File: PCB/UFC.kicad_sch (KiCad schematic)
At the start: 73 parts, among them M1 Fan_3pin, M2 Fan_3pin, M3 Fan_3pin, M4 Fan_3pin, M5 Fan_3pin, M6 Fan_3pin, M7 Fan_3pin, M8 Fan_3pin, SW1 PWM 12:5, U1 Pico

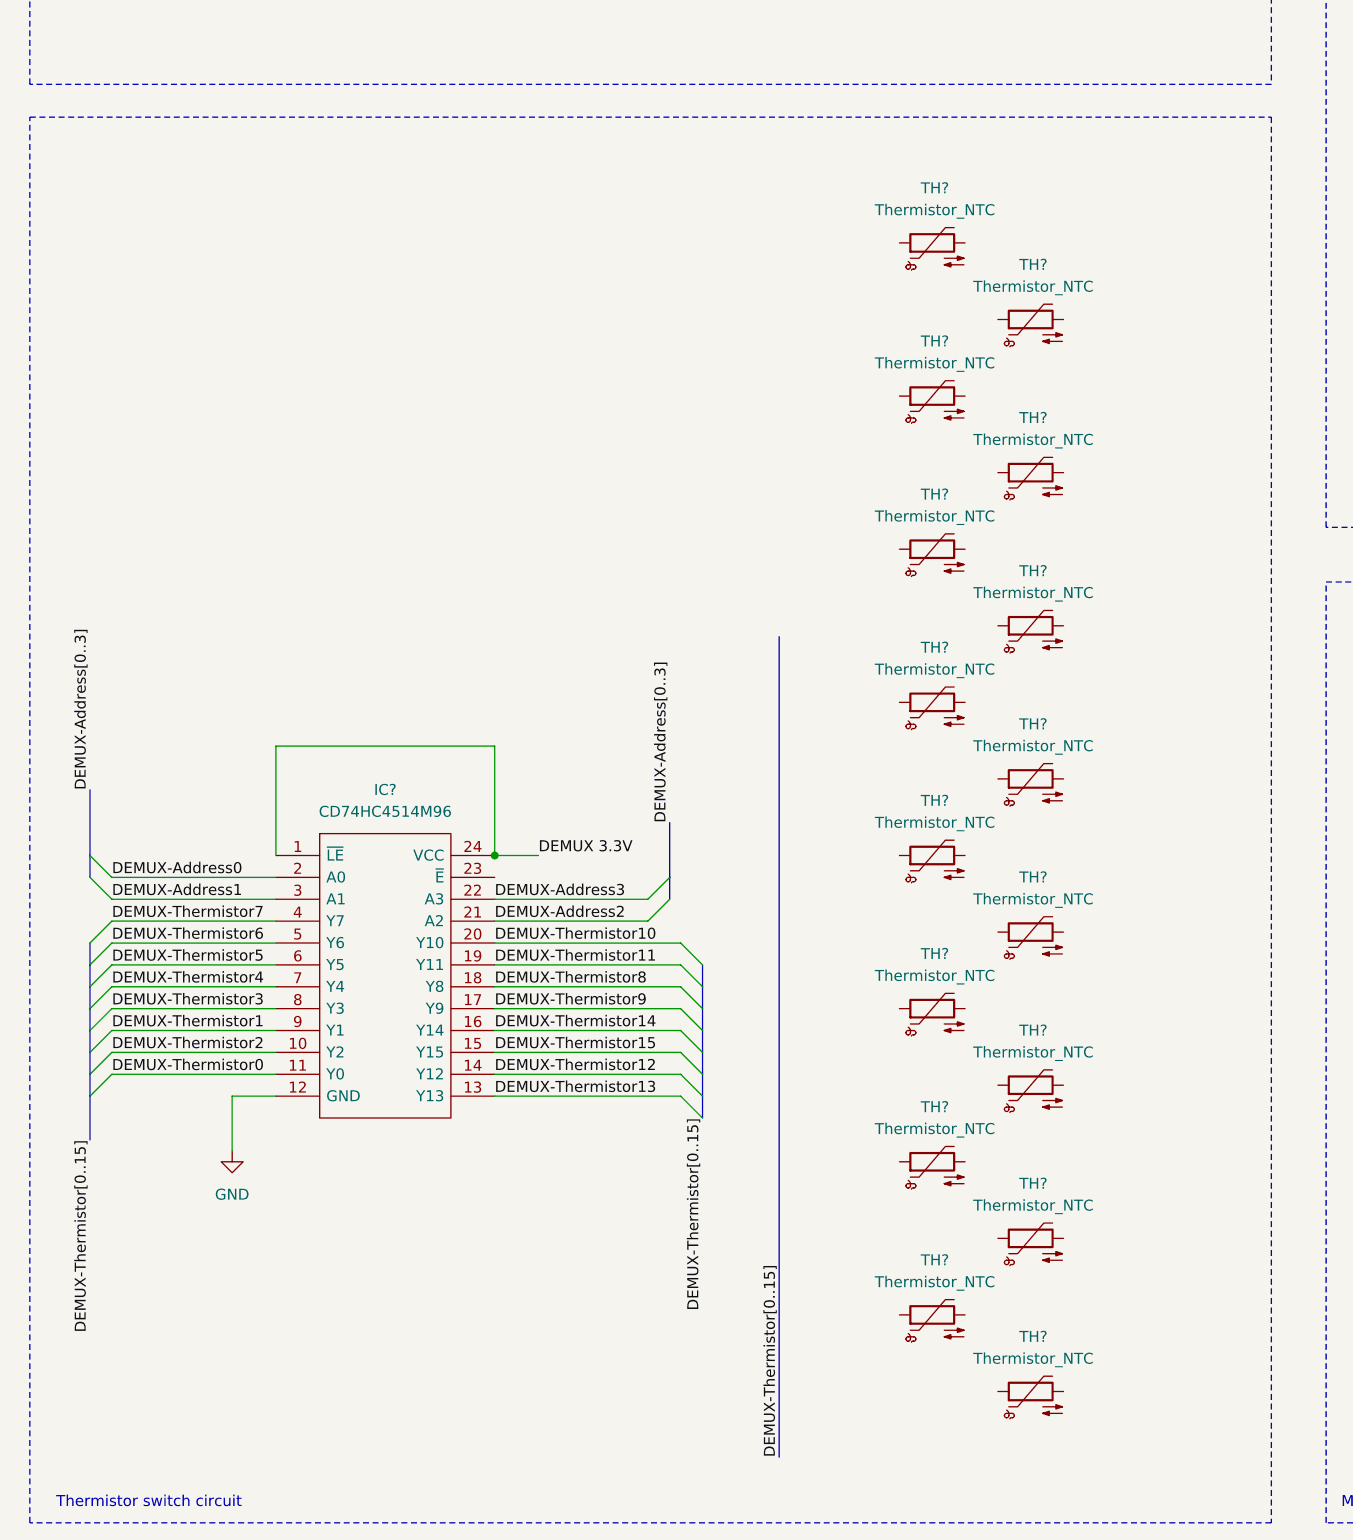
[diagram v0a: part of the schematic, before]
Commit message: update
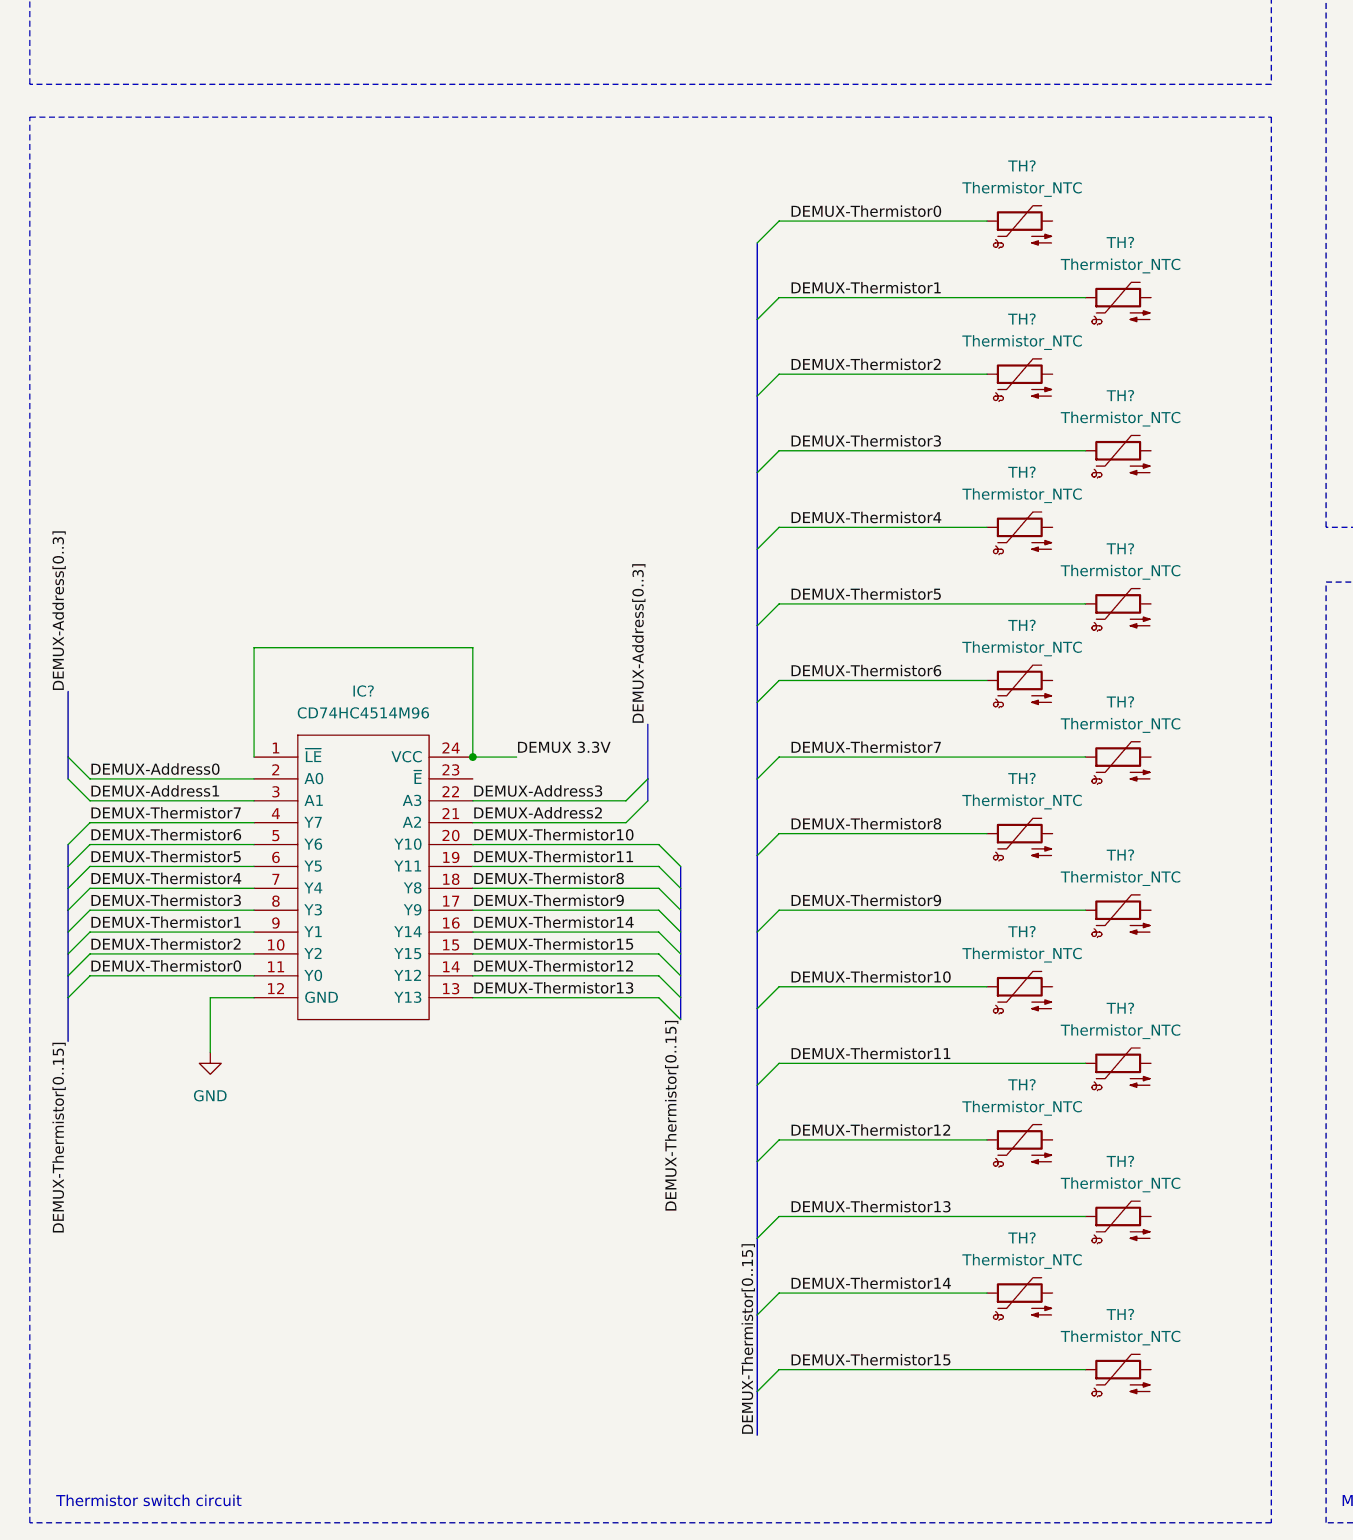
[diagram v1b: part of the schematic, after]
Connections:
- net DEMUX-Thermistor0: now also TH?.1
- net DEMUX-Thermistor1: now also TH?.1
- net DEMUX-Thermistor10: now also TH?.1
- net DEMUX-Thermistor11: now also TH?.1
- net DEMUX-Thermistor12: now also TH?.1
- net DEMUX-Thermistor13: now also TH?.1
- net DEMUX-Thermistor14: now also TH?.1
- net DEMUX-Thermistor15: now also TH?.1
- net DEMUX-Thermistor2: now also TH?.1
- net DEMUX-Thermistor3: now also TH?.1
- net DEMUX-Thermistor4: now also TH?.1
- net DEMUX-Thermistor5: now also TH?.1
- net DEMUX-Thermistor6: now also TH?.1
- net DEMUX-Thermistor7: now also TH?.1
- net DEMUX-Thermistor8: now also TH?.1
- net DEMUX-Thermistor9: now also TH?.1
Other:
- moved on the sheet: IC?, TH?
